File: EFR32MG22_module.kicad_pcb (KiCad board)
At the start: 2 copper layers, 29.9 x 42 mm, 34 parts, among them J1 USB_B_Micro 10118194-0011LF, J2 Conn_01x10, J3 Conn_ARM_JTAG_SWD_10, J4 Conn_01x10, U1 EFR32MG22C224F512GN32, U2 TLV75533PDBV, Y1 Crystal ECS-384-CDX-1983-TR3

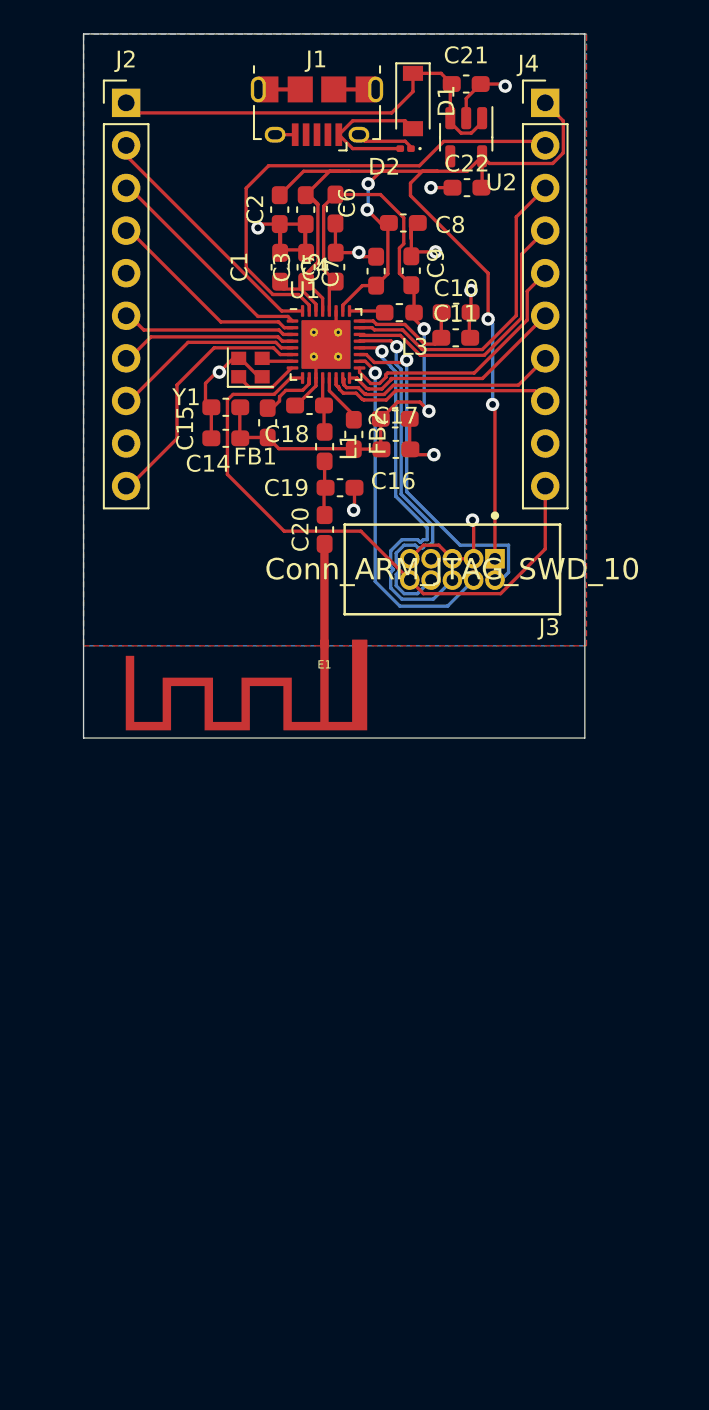
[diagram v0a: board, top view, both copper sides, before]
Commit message: final commit? (?)
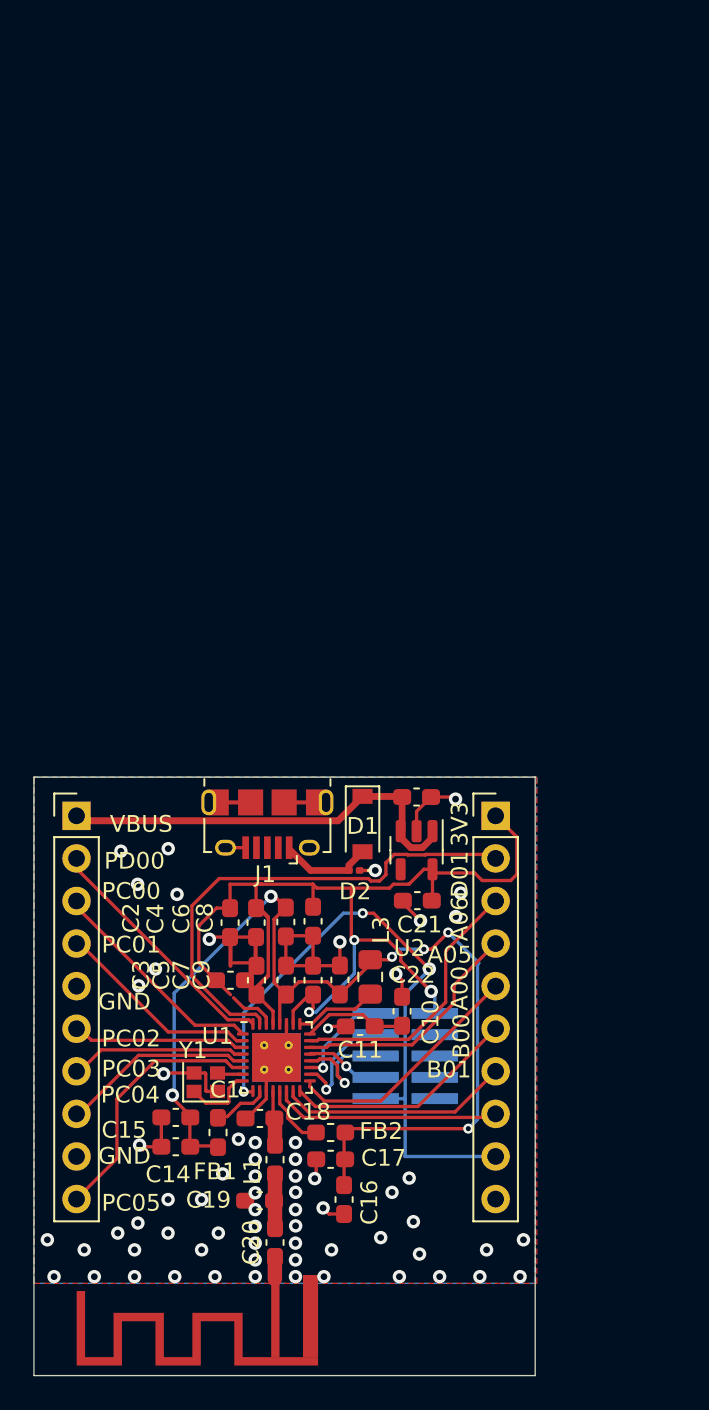
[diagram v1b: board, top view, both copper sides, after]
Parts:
- J3: value Conn_ARM_JTAG_SWD_10 -> ARM_2x5; footprint ARM_DEBUG:CNC_Tech_2x5_ARM_DEBUG -> arm_2x5:322010030000TR; moved to B.Cu
- L3: footprint Inductor_SMD:L_0603_1608Metric_Pad1.05x0.95mm_HandSolder -> Inductor_SMD:L_0805_2012Metric_Pad1.15x1.40mm_HandSolder
- moved C16 44.9 mm to (230.5, 149.5), turned to -90 degrees
- moved C17 44.3 mm to (229.7, 147.1), turned to 180 degrees
- moved D1 43.2 mm to (231.6, 127.1)
- moved D2 43.2 mm to (231.2, 129.9)
- moved C19 42.8 mm to (225.5, 149.6), turned to 180 degrees
- moved Y1 42.7 mm to (222.3, 142.5)
- moved L1 42.6 mm to (226.4, 147.1)
- moved C18 42.6 mm to (225.5, 144.7)
- moved C20 42.6 mm to (226.4, 152.1)
- moved C21 42.6 mm to (234.9, 125.5)
- moved C5 42.6 mm to (227.1, 136.4)
- moved C6 42.6 mm to (227.1, 133.0)
- moved J1 42.6 mm to (226.0, 127.1)
- moved J2 42.6 mm to (214.6, 126.6)
- moved J4 42.6 mm to (239.6, 126.6)
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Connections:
- J4 pad 10: /RESET_N -> GND
- J4 pad 9: GND -> /RESET_N
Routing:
- net VBUS: track 25.1 -> 48.1 mm
- net /DVDD: track 39.7 -> 62.7 mm, vias 2 -> 6
- net /TDI: track 22.2 -> 4.52 mm
- net /SWO: track 23.1 -> 6.89 mm
- net /SWDIO: track 20.7 -> 4.90 mm
- net /SWDCLK: track 20.8 -> 5.64 mm
- net +3.3V: track 75.5 -> 66.0 mm, vias 4 -> 3
- net GND: track 55.1 -> 45.7 mm, vias 10 -> 67
- net Net-(C20-Pad1): track 5.95 -> 1.31 mm
- net Net-(D1-Pad2): track 8.97 -> 5.55 mm
- net Net-(L3-Pad1): track 2.00 -> 4.93 mm
- net /RESET_N: track 36.2 -> 39.1 mm, vias 0 -> 3
- net /PA06: track 19.1 -> 16.3 mm
- net /PA05: track 16.9 -> 14.3 mm
- net /PAVDD: track 2.82 -> 3.90 mm
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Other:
- board size 29.9 x 42 mm -> 29.9 x 35.7 mm
- board text added: "3V3"
- board text added: "A moderately crappy Zigbee module"
- board text added: "A00"
- board text added: "A05"
- board text added: "A06"
- board text added: "B00"
- board text added: "B01"
- board text added: "D01"
- board text added: "GND"
- board text added: "PC00"
- board text added: "PC01"
- board text added: "PC02"
- board text added: "PC03"
- board text added: "PC04"
- board text added: "PC05"
- board text added: "PD00"
- board text added: "VBUS"
- board text added: "github.com/justchen1369"
- board text added: "{ "ViaStitching": "0.1", "stitch_zone_0": { "HSpacing": "1.27", "VSpacing": "1.27", "Clearance": "0.2", "Randomize": false }, "stitch_zone_1": { "HSpacing": "1", "VSpacing": "1", "Clearance": "0", "Randomize": false } }"
